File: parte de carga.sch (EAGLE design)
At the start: 42 parts, among them IC1 MCP73831T-2ACI_OT, IC10 741G3157DBVR, IC15 LMV321AIDCKR, IC16 LMV321AIDCKR, IC2 ESP32-S3-WROOM-1-N16R2, IC3 LMV321AIDCKR, IC5 LMV321AIDCKR, IC7 AD8226ARZ, IC9 LP38692MP-3.3_NOPB, J1 USB3500-30-A-KIT, J3 SJ-3523-SMT-TR, J4 1769

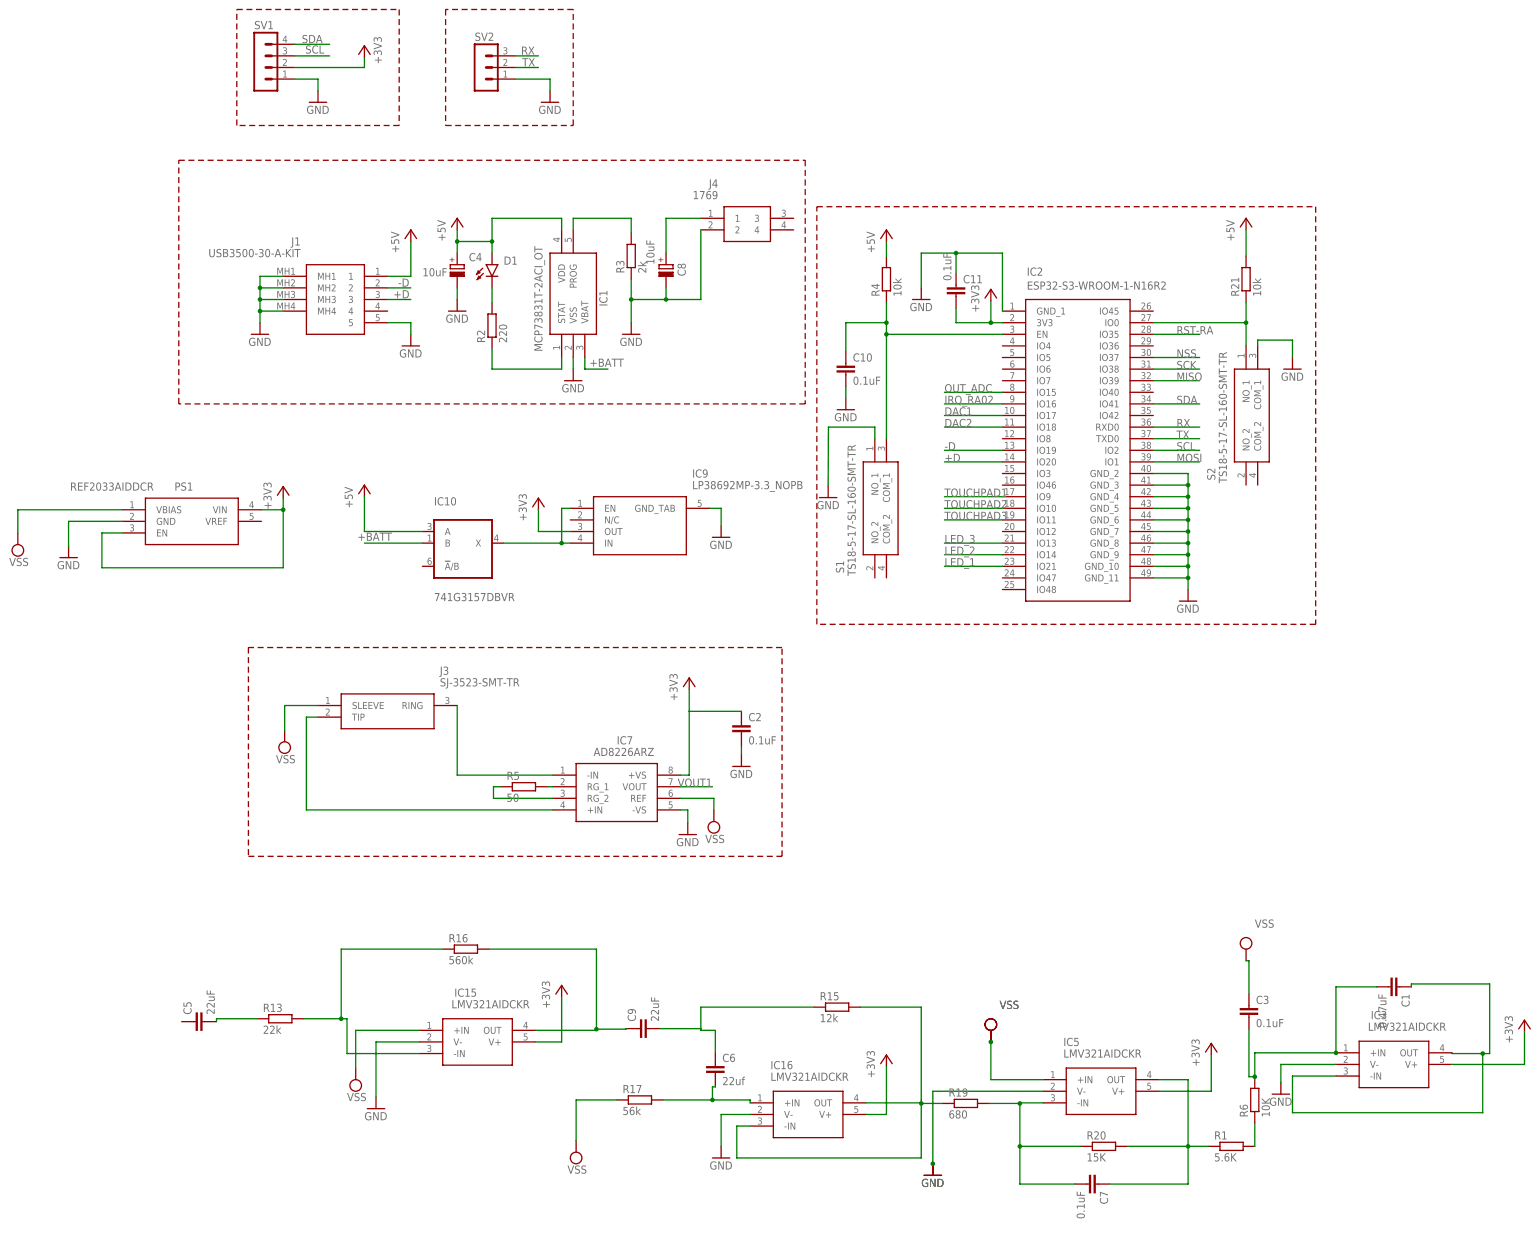
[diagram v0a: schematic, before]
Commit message: Astudillo estuvo aqui
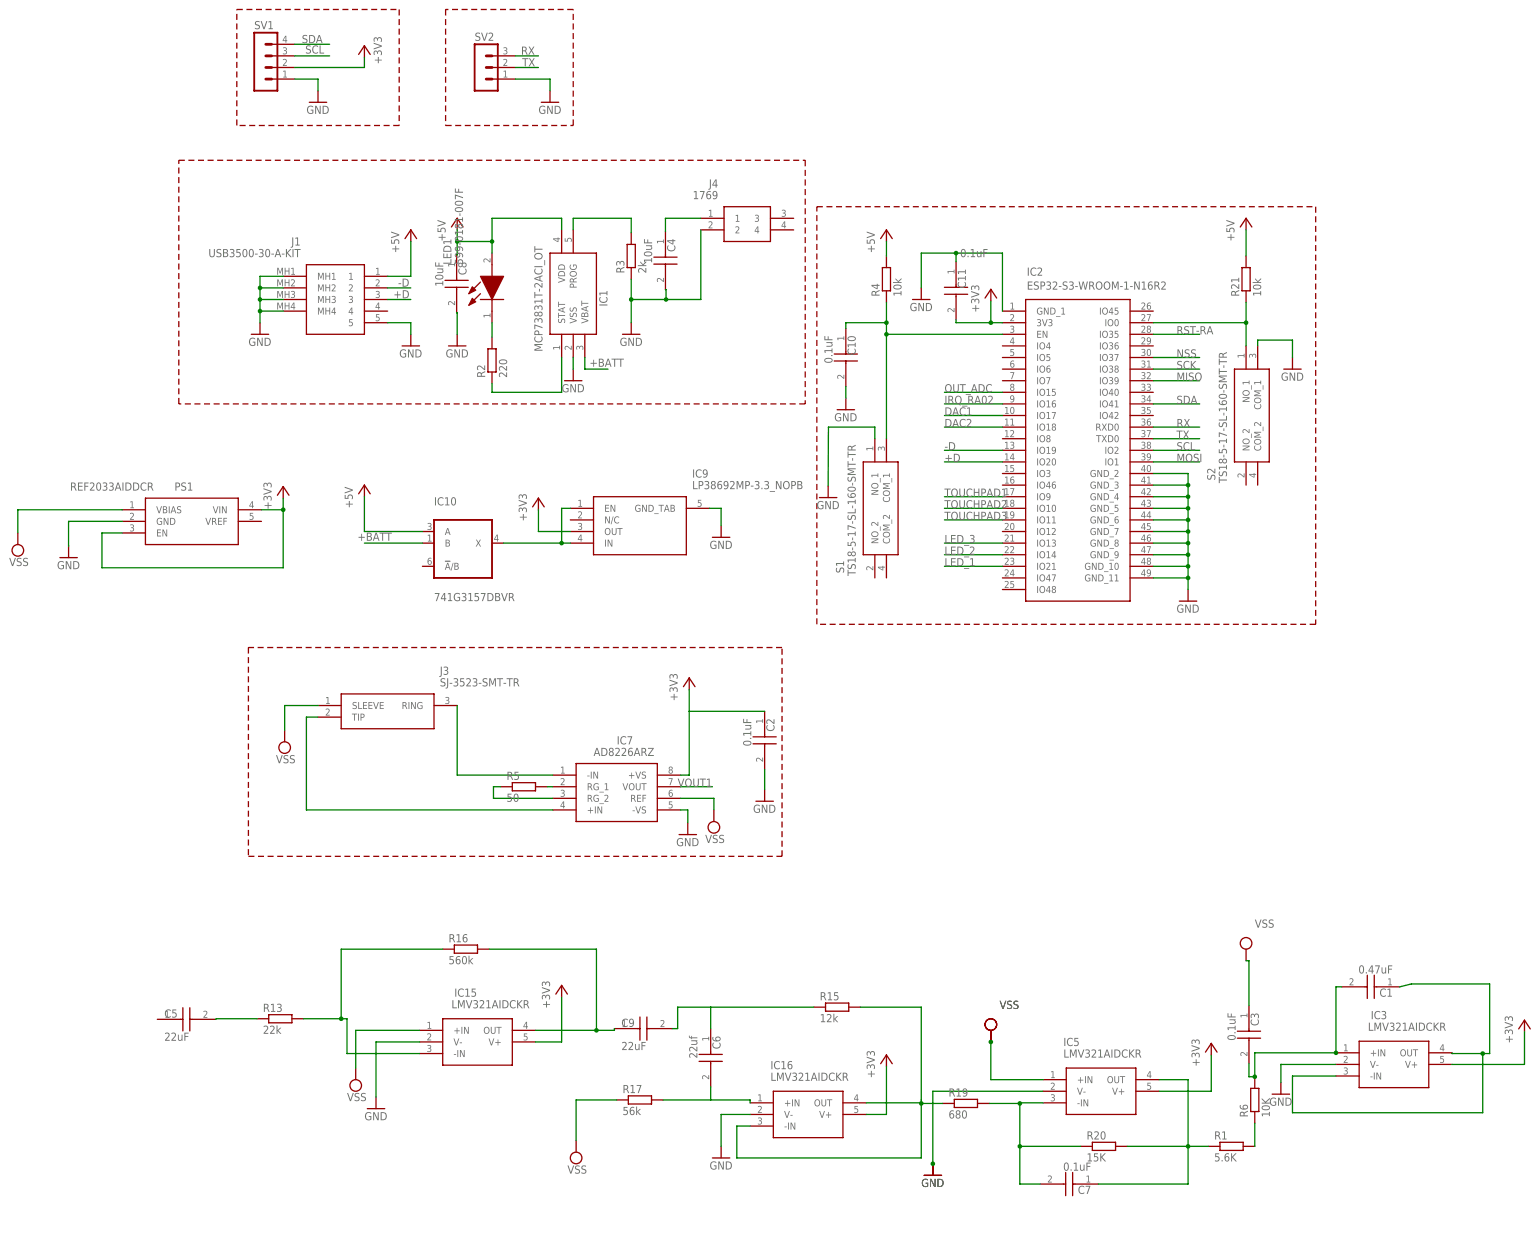
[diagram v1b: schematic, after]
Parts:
- removed D1: CHIP-FLAT-G_0603-0.35MM, LED:CHIP-FLAT-G_0603-0.35MM
- added LED1: 599-0181-007F, 599-0181-007F:599-0181-007F
- C1, C10, C11, C2, C3, C6, C7: device capacitor-wima:C2.5/5 -> GCM21B5C2A393JE02L:GCM21B5C2A393JE02L
- C4, C8: device Capacitor:C-POL_TANTALUM-1206(3216-METRIC) -> GCM21B5C2A393JE02L:GCM21B5C2A393JE02L
- C5, C9: device capacitor-wima:C2.5/5 -> GCM21B5C2A393JE02L:GCM21B5C2A393JE02L; POPULARITY 22uf -> (none)
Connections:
- removed net N$1 (its old number): D1.C, R2.2
- new net N$2: LED1.K, R2.2
- net +5V: now also C8.1, LED1.A; no longer C4.+, D1.A
- net GND: now also C4.2, C8.2; no longer C4.-, C8.-
- net N$19: now also C4.1; no longer C8.+
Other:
- moved on the sheet: R2
